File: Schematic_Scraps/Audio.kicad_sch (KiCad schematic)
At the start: 3 parts, among them U14 КР580ВИ53/8253, U8 КР1533ЛА3/74LS00

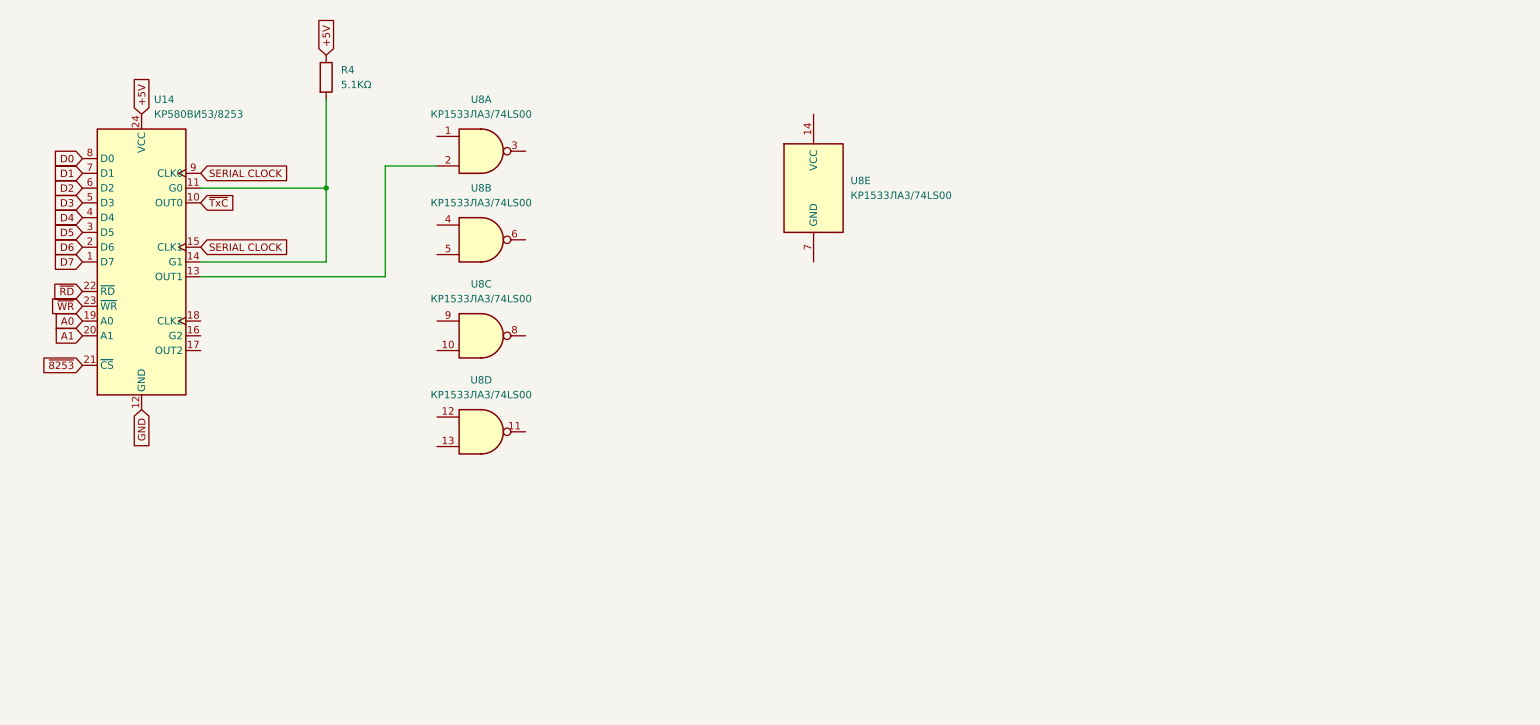
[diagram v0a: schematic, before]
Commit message: Further reverse engineering progress
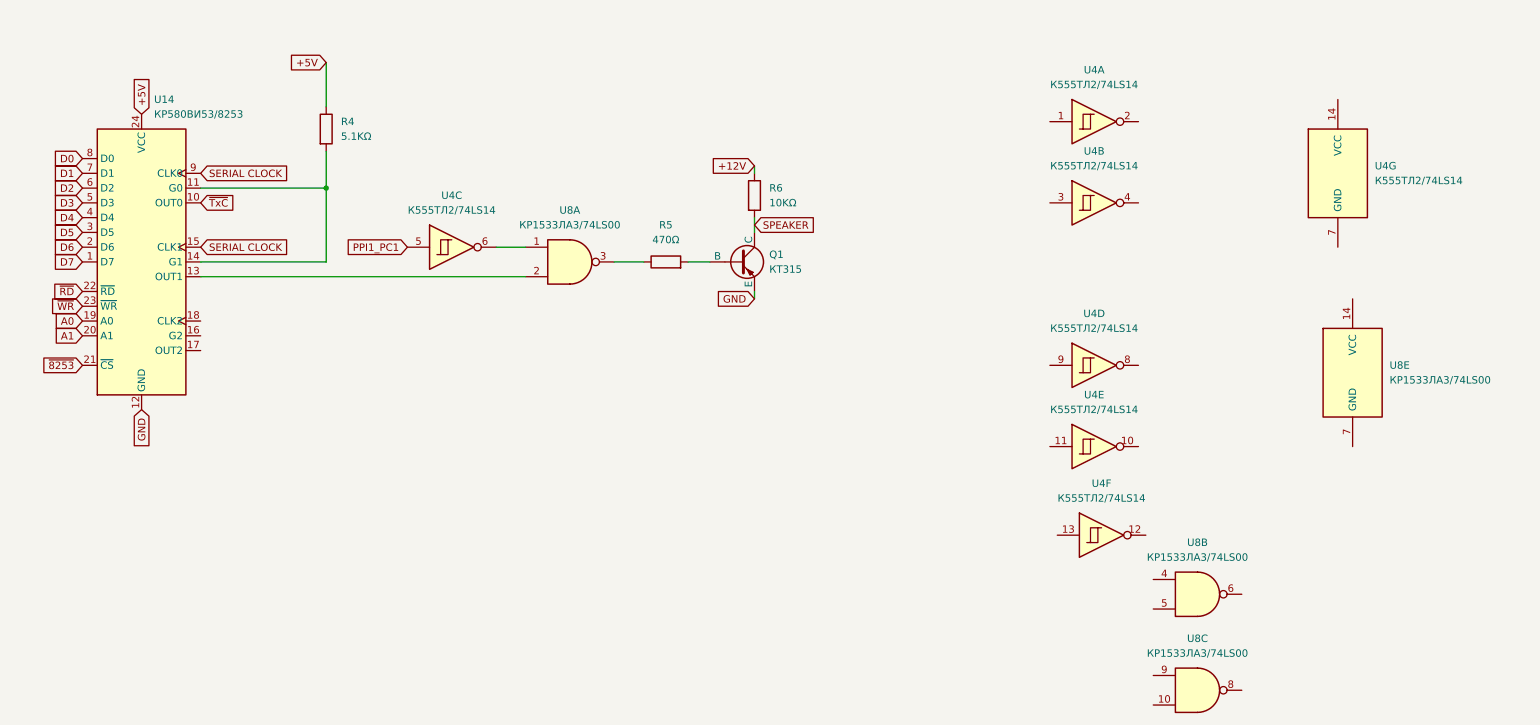
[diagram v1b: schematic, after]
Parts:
- removed unit 4 of U8
- added Q1: КТ315, symbol Simulation_SPICE:PNP
- added R5: 470Ω, symbol Device:R
- added R6: 10KΩ, symbol Device:R
- added U4: К555ТЛ2/74LS14, symbol 74xx:74LS14
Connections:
- net GND: now also Q1.3 (E)
- net at U8.1: now also U4.6
- net at U8.3: now also R5.1
- new net: Q1.2 (B), R5.2
- new net +12V: R6.1
- new net PPI1_PC1: U4.5
- new net SPEAKER: Q1.1 (C), R6.2
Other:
- company: (none) -> Brett Hallen
- title: (none) -> Rhythm Keyboard (Ритм Клав)
- moved on the sheet: R4, U8A, U8B, U8C, U8E

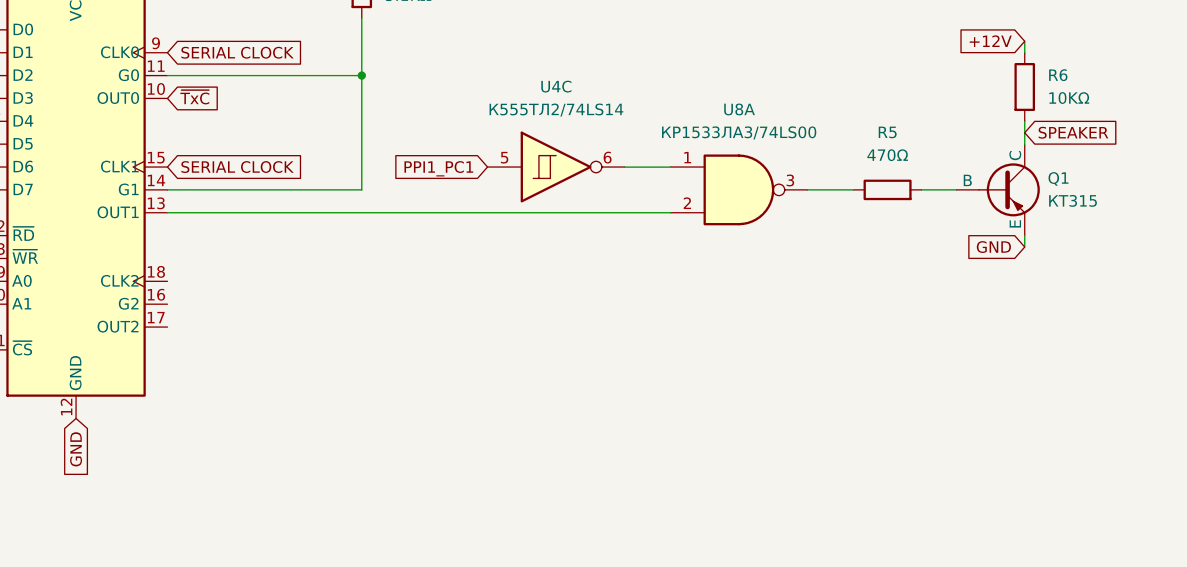
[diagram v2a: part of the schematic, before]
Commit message: 19-May reverse engineering progress
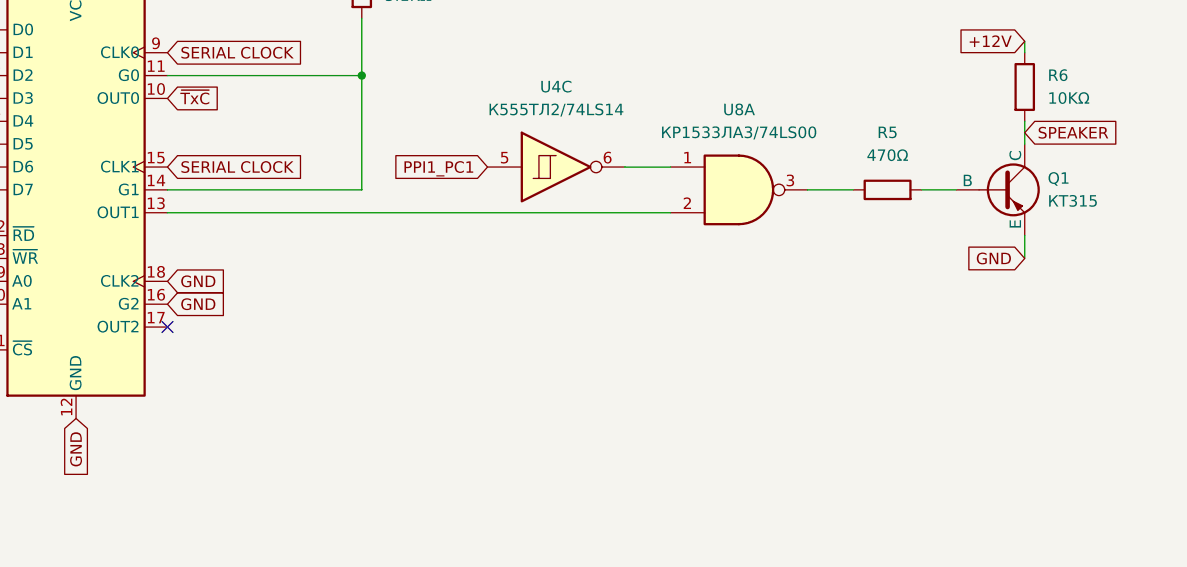
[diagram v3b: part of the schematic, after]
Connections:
- net GND: now also U14.16 (G2), U14.18 (CLK2)
- no-connect marks 0 -> 1
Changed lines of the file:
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@@
 	(generator "eeschema")
 	(generator_version "9.0")
-	(paper "A4")
+	(paper "A3")
 	(title_block
 		(title "Rhythm Keyboard (Ритм Клав)")
@@
 		(color 0 0 0 0)
 	)
+	(no_connect
+		(at 73.66 73.66)
+	)
 	(wire
 		(pts
@@
 	(wire
 		(pts
-			(xy 168.91 64.77) (xy 168.91 63.5)
+			(xy 168.91 66.04) (xy 168.91 63.5)
 		)
 		(stroke
@@
 		)
 	)
+	(global_label "GND"
+		(shape input)
+		(at 73.66 71.12 0)
+		(fields_autoplaced yes)
+		(effects
+			(font
+				(size 1.27 1.27)
+			)
+			(justify left)
+		)
+		(property "Intersheetrefs" "${INTERSHEET_REFS}"
+			(at 80.5157 71.12 0)
+			(effects
+				(font
+					(size 1.27 1.27)
+				)
+				(justify left)
+				(hide yes)
+			)
+		)
+	)
 	(global_label "D4"
 		(shape input)
@@
 	(global_label "GND"
 		(shape input)
-		(at 168.91 64.77 180)
-		(fields_autoplaced yes)
-		(effects
-			(font
-				(size 1.27 1.27)
-			)
-			(justify right)
-		)
-		(property "Intersheetrefs" "${INTERSHEET_REFS}"
-			(at 162.0543 64.77 0)
+		(at 168.91 66.04 180)
+		(fields_autoplaced yes)
+		(effects
+			(font
+				(size 1.27 1.27)
+			)
+			(justify right)
+		)
+		(property "Intersheetrefs" "${INTERSHEET_REFS}"
+			(at 162.0543 66.04 0)
 			(effects
 				(font
@@
 				(hide yes)
 			)
+		)
+	)
+	(global_label "GND"
+		(shape input)
+		(at 73.66 68.58 0)
+		(fields_autoplaced yes)
+		(effects
+			(font
+				(size 1.27 1.27)
+			)
+			(justify left)
+		)
+		(property "Intersheetrefs" "${INTERSHEET_REFS}"
+			(at 80.5157 68.58 0)
+			(effects
+				(font
+					(size 1.27 1.27)
+				)
+				(justify left)
+				(hide yes)
+			)
